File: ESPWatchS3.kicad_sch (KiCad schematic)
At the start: 113 parts, among them J1 OLED, J2 USB, J3 UART0, U1 ESP32-S3R8, U10 BD48KxxG, U2 EVA-M8Q-0, U3 BME280, U4 IS25LP128F-JKLE, U5 BQ27441-G1A, U6 BQ24075RGTR, U7 TPS631000DRLR, U8 AP3012, U9 NJG1143UA2-TE1, Y1 40MHz, Y2 32.768kHz, Y3 32.768kHz

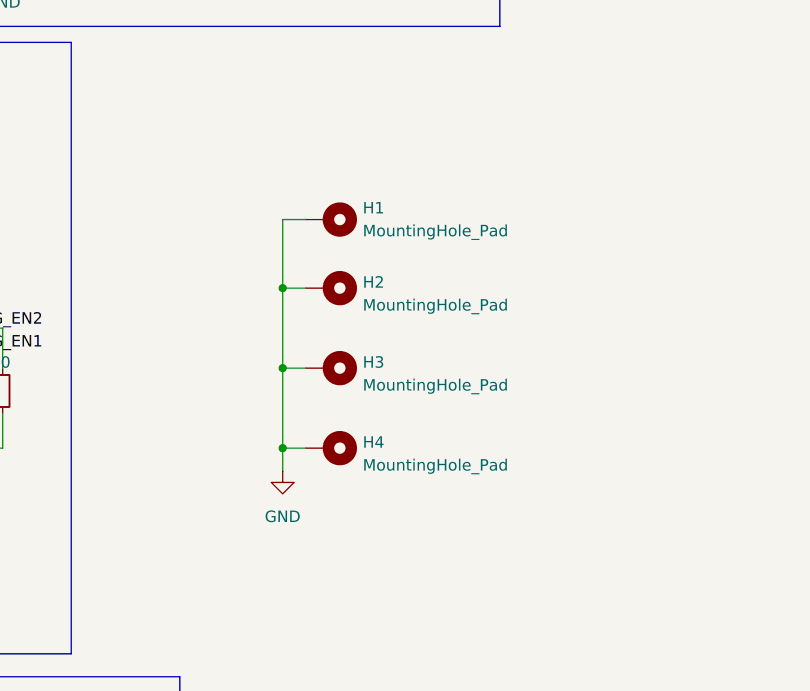
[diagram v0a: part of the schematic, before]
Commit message: PCB Work
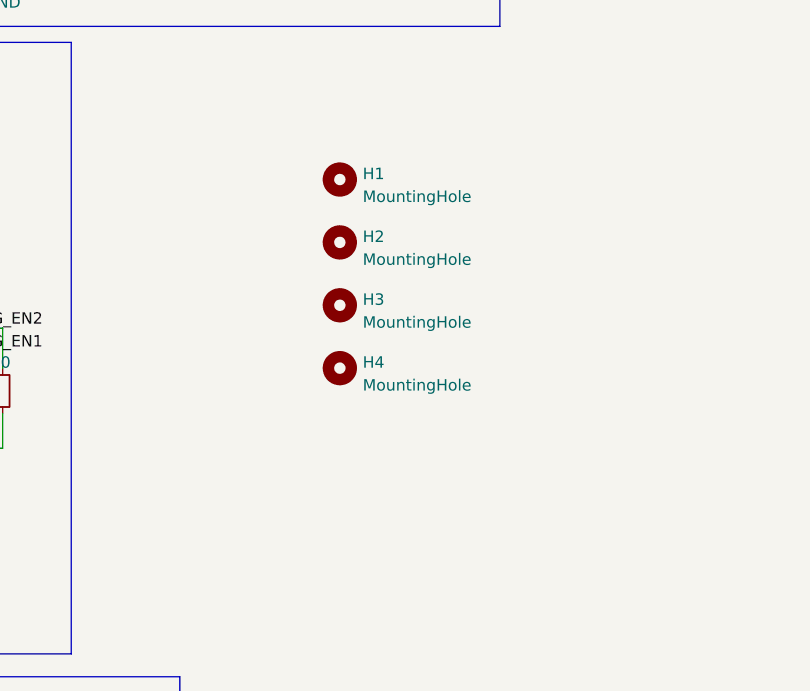
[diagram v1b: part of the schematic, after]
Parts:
- removed H1, H2, H3, H4: MountingHole_Pad, MountingHole:MountingHole_2.2mm_M2_Pad, symbol Mechanical:MountingHole_Pad
- added H1, H2, H3, H4: MountingHole, MountingHole:MountingHole_2.2mm_M2, symbol Mechanical:MountingHole
